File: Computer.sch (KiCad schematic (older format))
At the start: 35 parts, among them J1 DB9, J2 Screw_Terminal_1x04, U1 8284, U10 74LS04, U11 7400, U12 8259, U2 LM2931AZ-5.0, U3 8088, U4 74LS04, U5 28C256, U6 RAM_32KO, U7 16450, U8 7400, U9 NCP1117DT12G, Y1 8 MHz, Y2 3.072 MHz

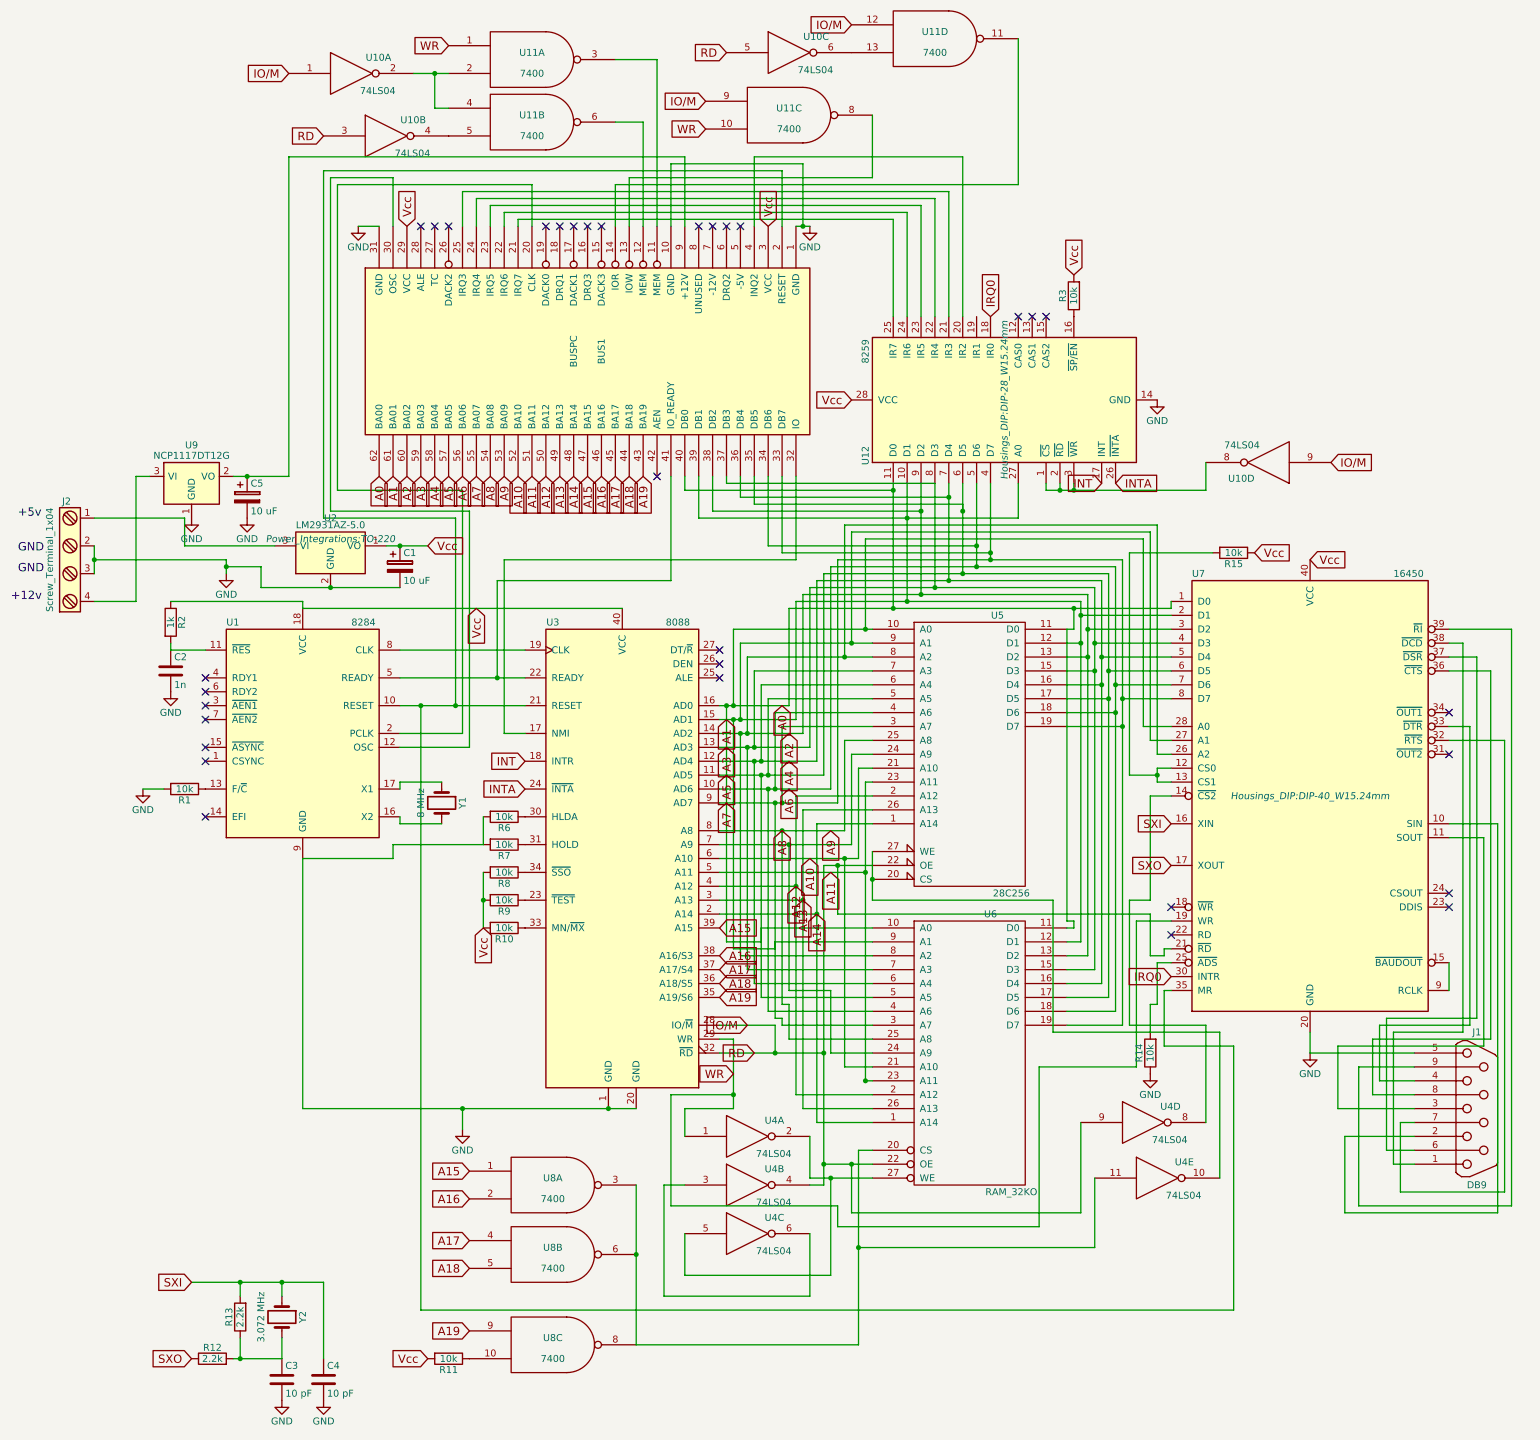
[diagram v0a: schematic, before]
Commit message: Update to revision A
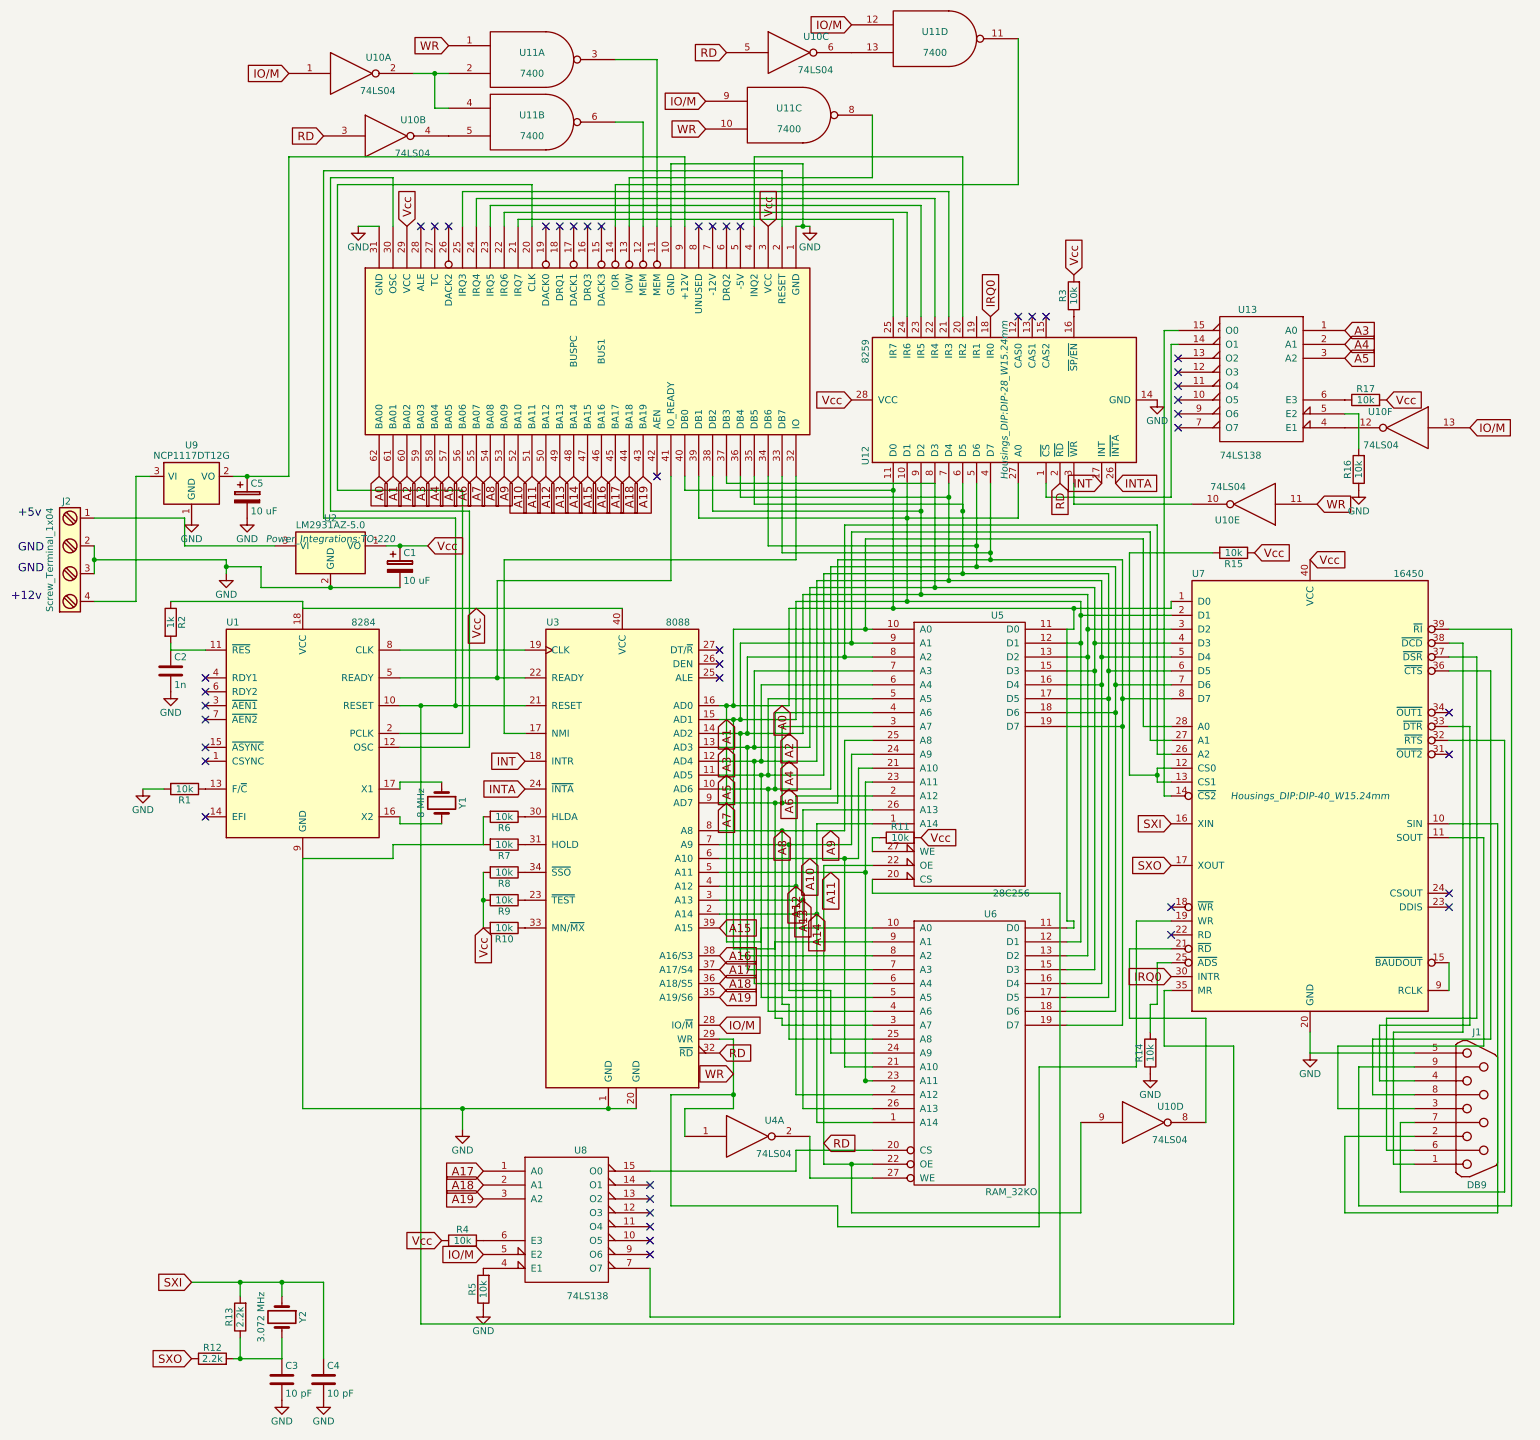
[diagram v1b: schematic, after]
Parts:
- removed unit 2 of U4
- removed unit 3 of U4
- removed unit 4 of U4
- removed unit 5 of U4
- removed U8: 7400, Housings_DIP:DIP-14_W7.62mm, symbol 7400
- added R16, R17, R4, R5: 10k, Resistors_THT:R_Axial_DIN0204_L3.6mm_D1.6mm_P7.62mm_Horizontal, symbol R
- added unit 6 of U10
- added unit 5 of U10
- added U13, U8: 74LS138, Housings_DIP:DIP-16_W7.62mm, symbol 74LS138
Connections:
- net A0: now also U13.1 (A0), U13.3 (A2)
- net A17: now also U8.1 (A0)
- net A18: now also U8.2 (A1)
- net A19: now also U8.3 (A2)
- net A4: now also U13.2 (A1)
- net GND: now also R16.1, R5.1, U10.7 (GND), U10.7 (GND), U13.8 (GND), U8.8 (GND)
- net IO/M: now also U10.13, U8.5 (E2); no longer U10.3, U10.5, U10.9, U3.32 (~RD~), U5.22 (OE), U6.22 (OE), U7.21 (~RD~)
- net VCC: now also U10.14 (VCC), U10.14 (VCC), U13.16 (VCC), U8.16 (VCC)
- net Vcc: now also R17.2, R4.1
- net WR: now also U10.11
- net at U5.20 (CS): now also U8.7 (O7); no longer U5.27 (WE)
- net at U6.20 (CS): now also U8.15 (O0)
- net at U7.14 (~CS2~): now also U13.15 (O0)
- net at R11.1: now also U5.27 (WE)
- new net: U10.8, U7.21 (~RD~)
- new net: U12.1 (~CS~), U13.14 (O1)
- new net: U10.10, U12.3 (~WR~)
- new net: R5.2, U8.4 (E1)
- new net: R4.2, U8.6 (E3)
- new net: U10.12, U13.4 (E1)
- new net: R16.2, U13.5 (E2)
- new net: R17.1, U13.6 (E3)
- new net RD: U10.3, U10.5, U10.9, U12.2 (~RD~), U3.32 (~RD~), U5.22 (OE), U6.22 (OE)
- no-connect marks 32 -> 44
